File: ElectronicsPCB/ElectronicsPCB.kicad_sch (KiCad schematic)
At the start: 36 parts

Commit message: order control pcb with these gerbers
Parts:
- 3.3V_SYS1, 5V_SYS1, ANEMOMETER1, CAMERA1, EXTRA1, EXTRA2, HEADERS1, SAIL1, StepDownChip1, TAIL1, TEENSY1, VectorNavInput1, XBEE1: now left out of the parts list
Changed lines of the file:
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@@
 		(unit 1)
 		(exclude_from_sim no)
-		(in_bom yes)
+		(in_bom no)
 		(on_board yes)
 		(dnp no)
@@
 		(unit 1)
 		(exclude_from_sim no)
-		(in_bom yes)
+		(in_bom no)
 		(on_board yes)
 		(dnp no)
@@
 		(unit 1)
 		(exclude_from_sim no)
-		(in_bom yes)
+		(in_bom no)
 		(on_board yes)
 		(dnp no)
@@
 		(unit 1)
 		(exclude_from_sim no)
-		(in_bom yes)
+		(in_bom no)
 		(on_board yes)
 		(dnp no)
@@
 		(unit 1)
 		(exclude_from_sim no)
-		(in_bom yes)
+		(in_bom no)
 		(on_board yes)
 		(dnp no)
@@
 		(unit 1)
 		(exclude_from_sim no)
-		(in_bom yes)
+		(in_bom no)
 		(on_board yes)
 		(dnp no)
@@
 		(unit 1)
 		(exclude_from_sim no)
-		(in_bom yes)
+		(in_bom no)
 		(on_board yes)
 		(dnp no)
@@
 		(unit 1)
 		(exclude_from_sim no)
-		(in_bom yes)
+		(in_bom no)
 		(on_board yes)
 		(dnp no)
@@
 		(unit 1)
 		(exclude_from_sim no)
-		(in_bom yes)
+		(in_bom no)
 		(on_board yes)
 		(dnp no)
@@
 		(unit 1)
 		(exclude_from_sim no)
-		(in_bom yes)
+		(in_bom no)
 		(on_board yes)
 		(dnp no)
@@
 		(unit 1)
 		(exclude_from_sim no)
-		(in_bom yes)
+		(in_bom no)
 		(on_board yes)
 		(dnp no)
@@
 		(unit 1)
 		(exclude_from_sim no)
-		(in_bom yes)
+		(in_bom no)
 		(on_board yes)
 		(dnp no)
@@
 		(unit 1)
 		(exclude_from_sim no)
-		(in_bom yes)
+		(in_bom no)
 		(on_board yes)
 		(dnp no)

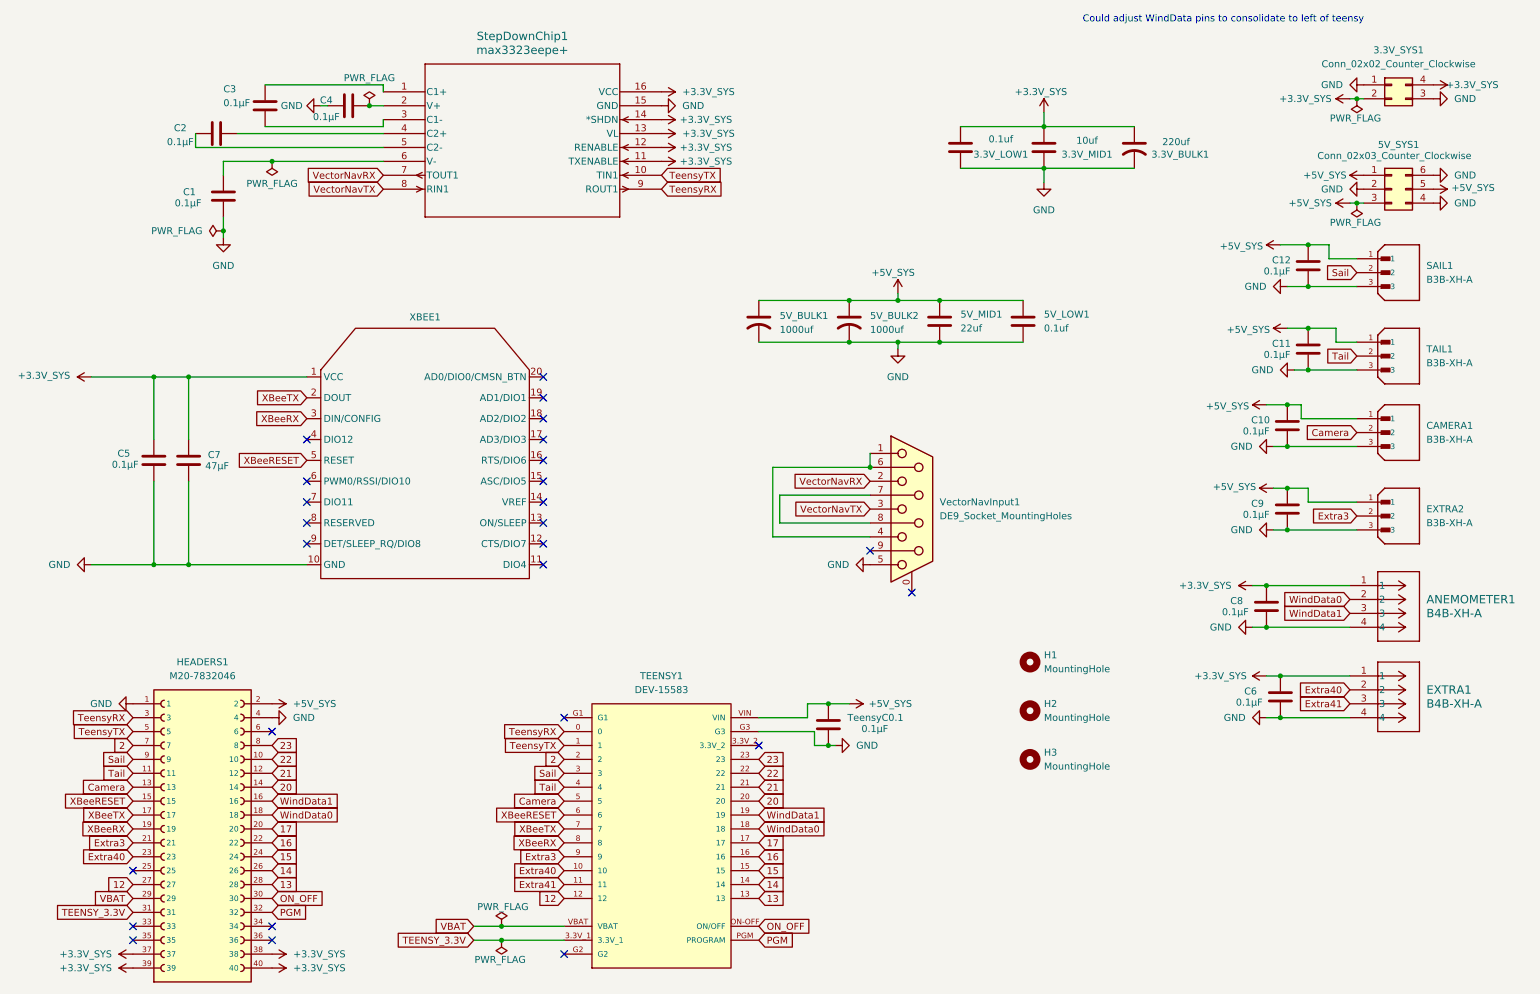
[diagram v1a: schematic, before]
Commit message: series of changes
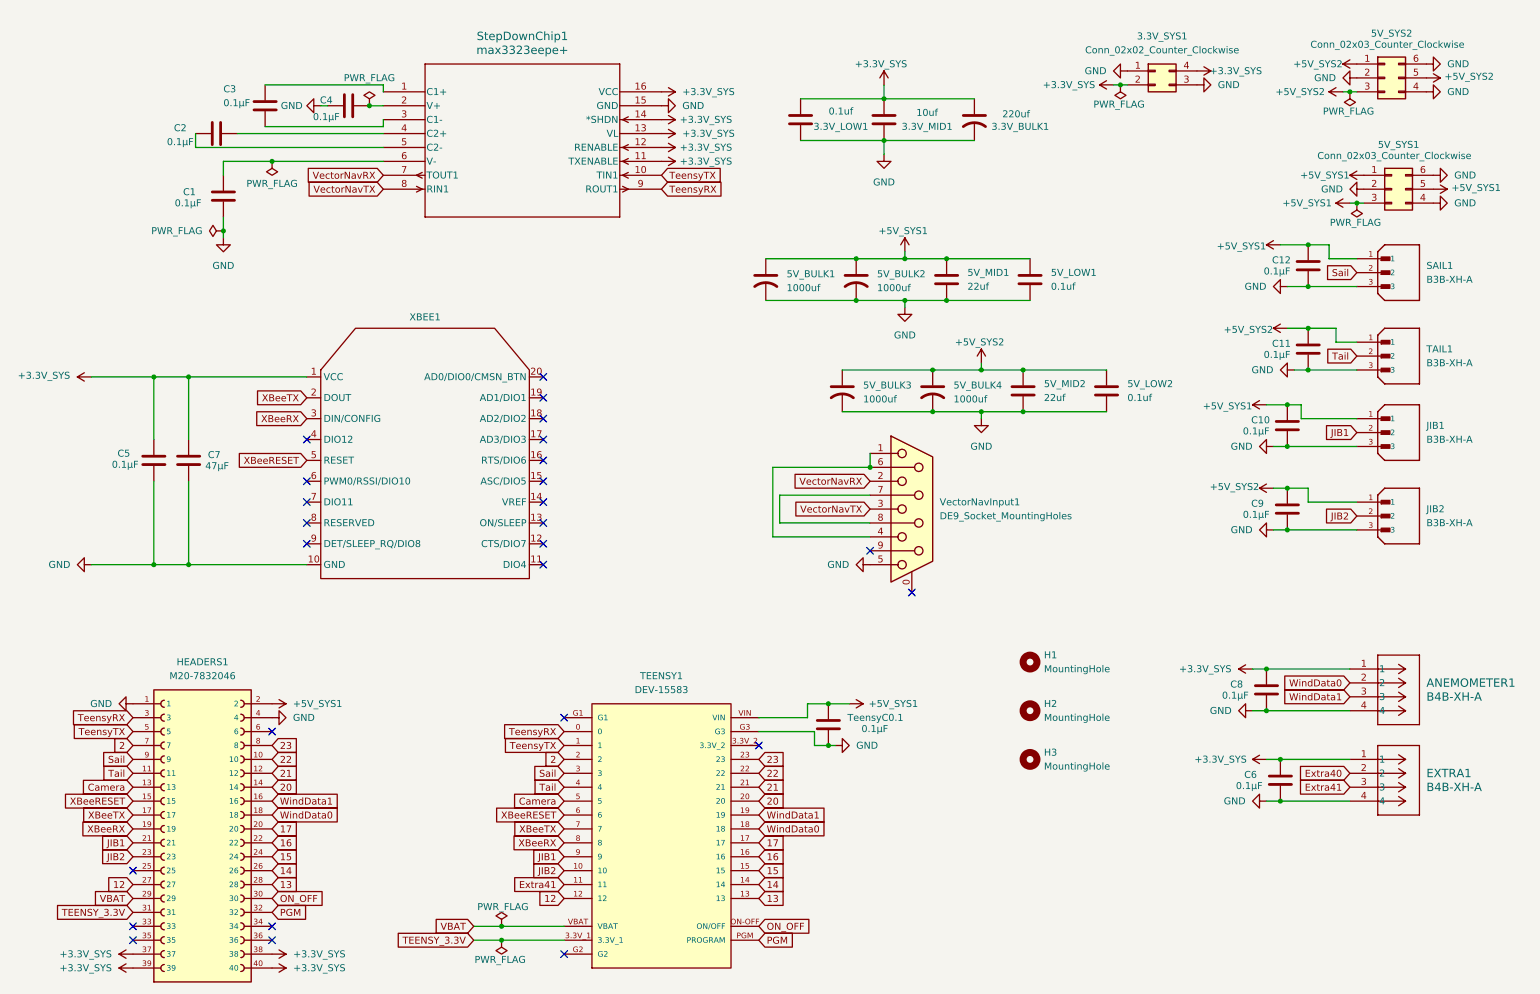
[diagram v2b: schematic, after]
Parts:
- added 5V_BULK3, 5V_BULK4: 1000uf, ElectronicsFootprints:CAP_EEE1A_1000uf, symbol Device:C_US
- added 5V_LOW2: 0.1uf, ElectronicsFootprints:CAP_CL10B_01uf_0603, symbol Device:C
- added 5V_MID2: 22uf, ElectronicsFootprints:CAP_CL32A_22uf_1210, symbol Device:C
- added 5V_SYS2: Conn_02x03_Counter_Clockwise, Connector_Molex:Molex_Mini-Fit_Jr_5566-06A_2x03_P4.20mm_Vertical, symbol Connector_Generic:Conn_02x03_Counter_Clockwise
- renumbered CAMERA1 to JIB1, EXTRA2 to JIB2
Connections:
- net Camera: no longer JIB1.2
- net Extra40: no longer HEADERS1.23, TEENSY1.10
- net GND: now also 5V_BULK3.2, 5V_BULK4.2, 5V_LOW2.1, 5V_MID2.1, 5V_SYS2.2 (Pin_2), 5V_SYS2.4 (Pin_4), 5V_SYS2.6 (Pin_6)
- net +5V_SYS renamed +5V_SYS1
- net +5V_SYS1: no longer C11.1, C9.1, JIB2.1, TAIL1.1
- net Extra3 renamed JIB1
- net JIB1: now also JIB1.2; no longer JIB2.2
- new net +5V_SYS2: 5V_BULK3.1, 5V_BULK4.1, 5V_LOW2.2, 5V_MID2.2, 5V_SYS2.1 (Pin_1), 5V_SYS2.3 (Pin_3), 5V_SYS2.5 (Pin_5), C11.1, C9.1, JIB2.1, TAIL1.1
- new net JIB2: HEADERS1.23, JIB2.2, TEENSY1.10
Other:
- note removed: "Could adjust WindData pins to consolidate to left of teensy"
- moved on the sheet: 3.3V_BULK1, 3.3V_LOW1, 3.3V_MID1, 3.3V_SYS1, 5V_BULK1, 5V_BULK2, 5V_LOW1, 5V_MID1, ANEMOMETER1, C6, C8, EXTRA1
